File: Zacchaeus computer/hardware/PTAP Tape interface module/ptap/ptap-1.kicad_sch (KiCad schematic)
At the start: 10 parts, among them J1 Conn_02x40_Top_Bottom, SW1 SW_DIP_x08, U1 74LS139, U2 74LS32, U3 74HCT688

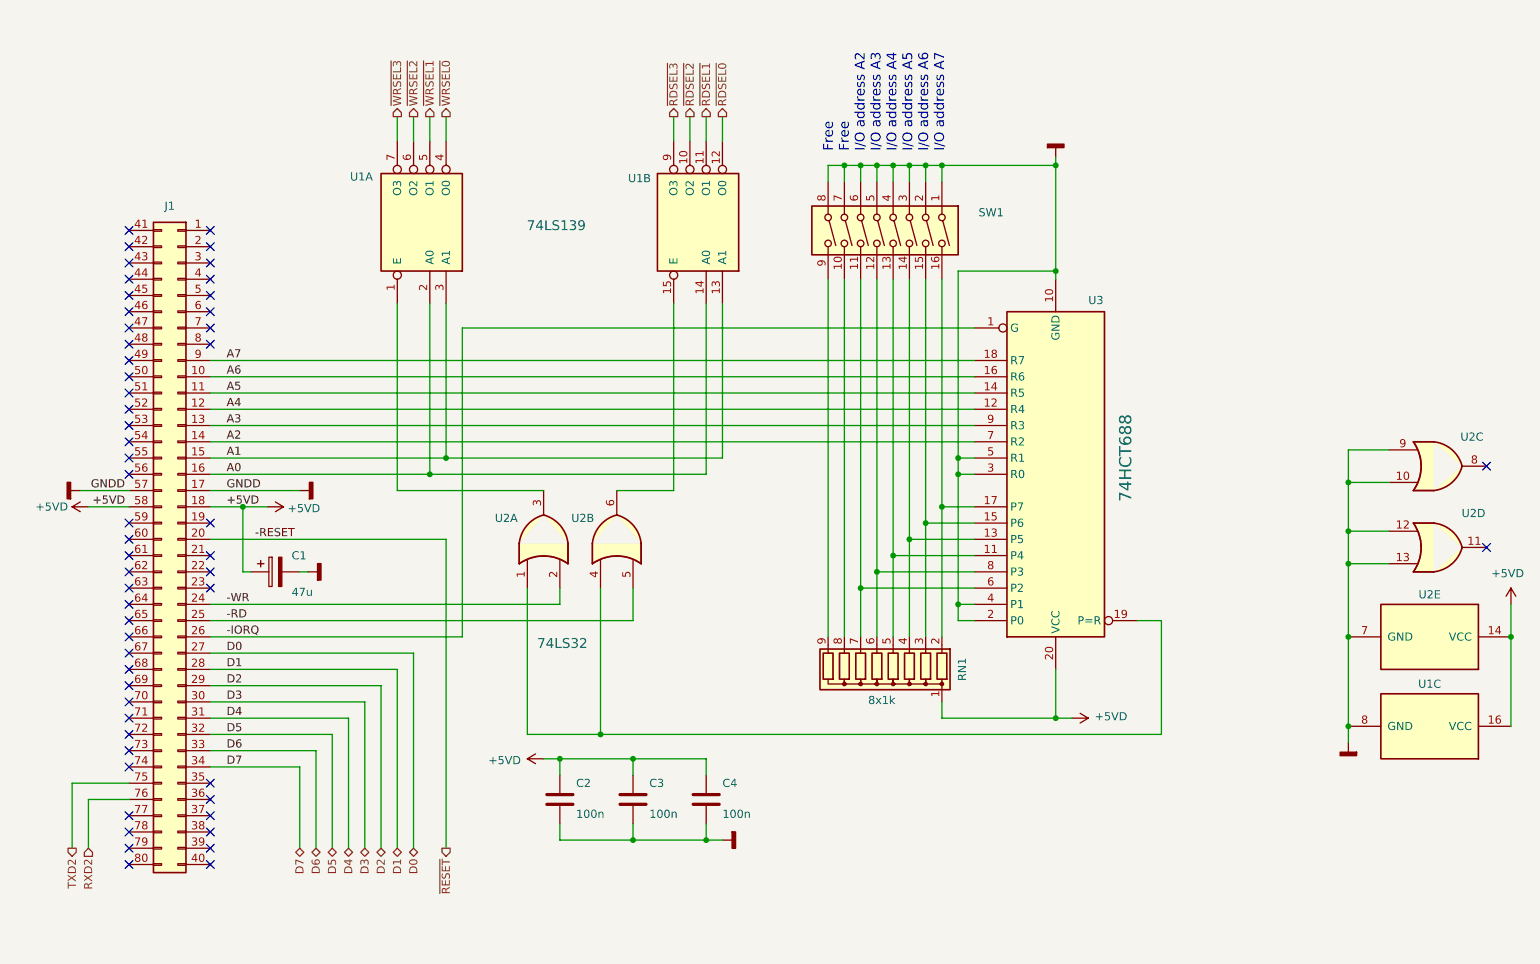
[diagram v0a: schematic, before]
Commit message: 260405
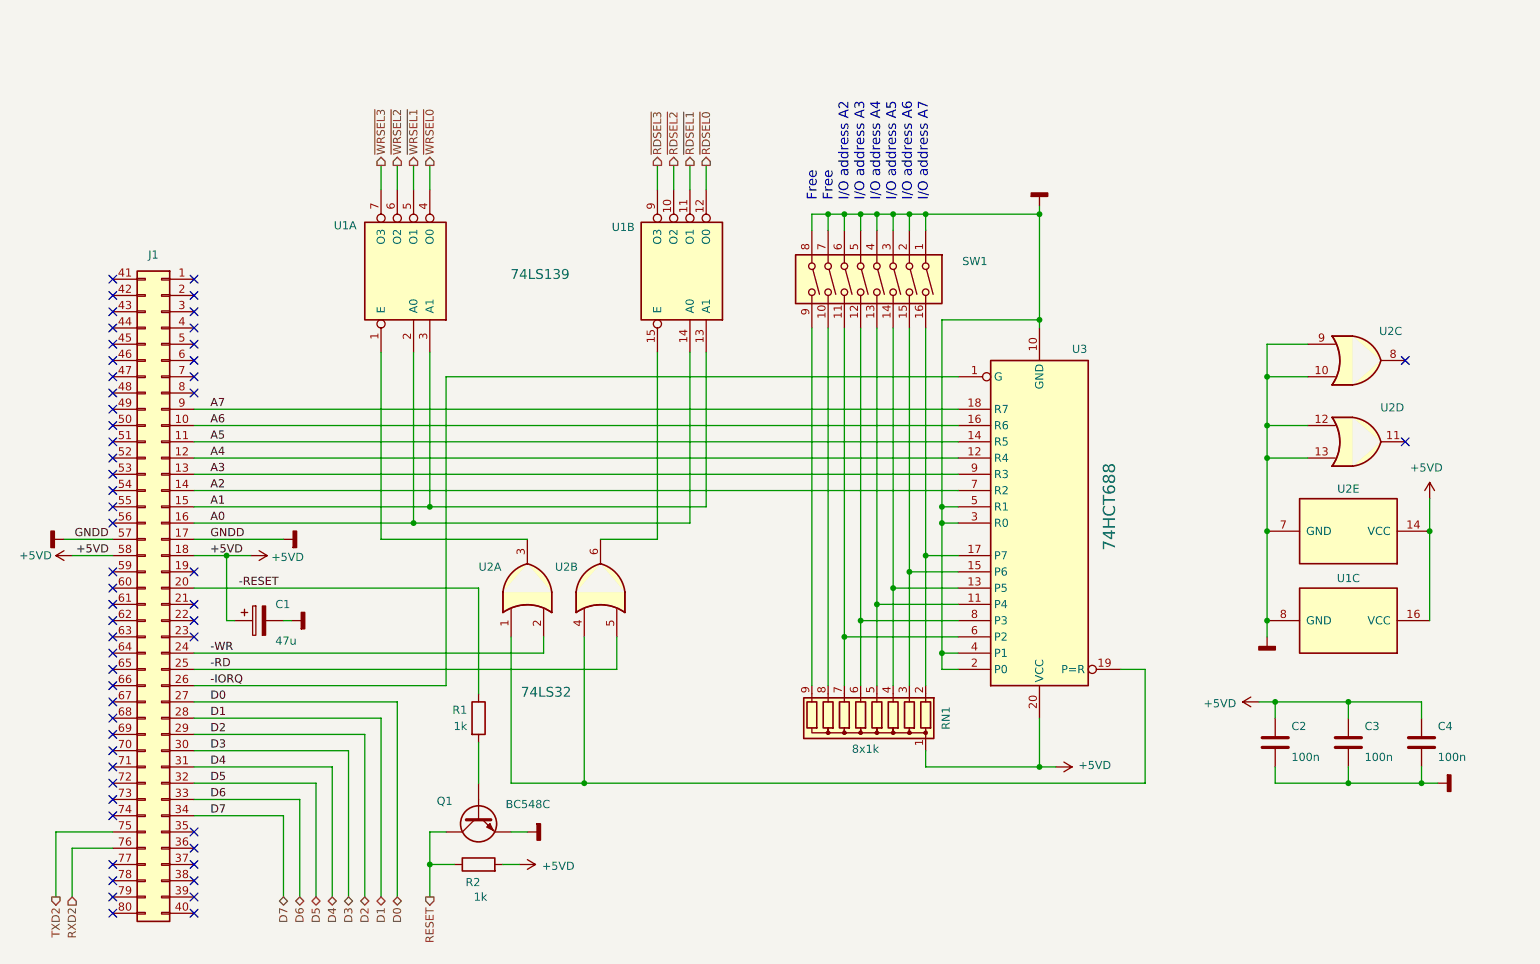
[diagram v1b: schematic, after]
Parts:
- added Q1: BC548C, symbol Simulation_SPICE:NPN
- added R1, R2: 1k, symbol Device:R
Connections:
- net +5VD: now also R2.2
- net GNDD: now also Q1.3 (E)
- net ~{RESET} renamed -RESET
- net -RESET: now also R1.1
- new net: Q1.2 (B), R1.2
- new net RESET: Q1.1 (C), R2.1
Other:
- moved on the sheet: C1, C2, C3, C4, J1, RN1, SW1, U1A, U1B, U1C, U2A, U2B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
